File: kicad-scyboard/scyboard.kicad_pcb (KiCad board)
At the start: 2 copper layers, 149 x 95.4 mm, 92 parts

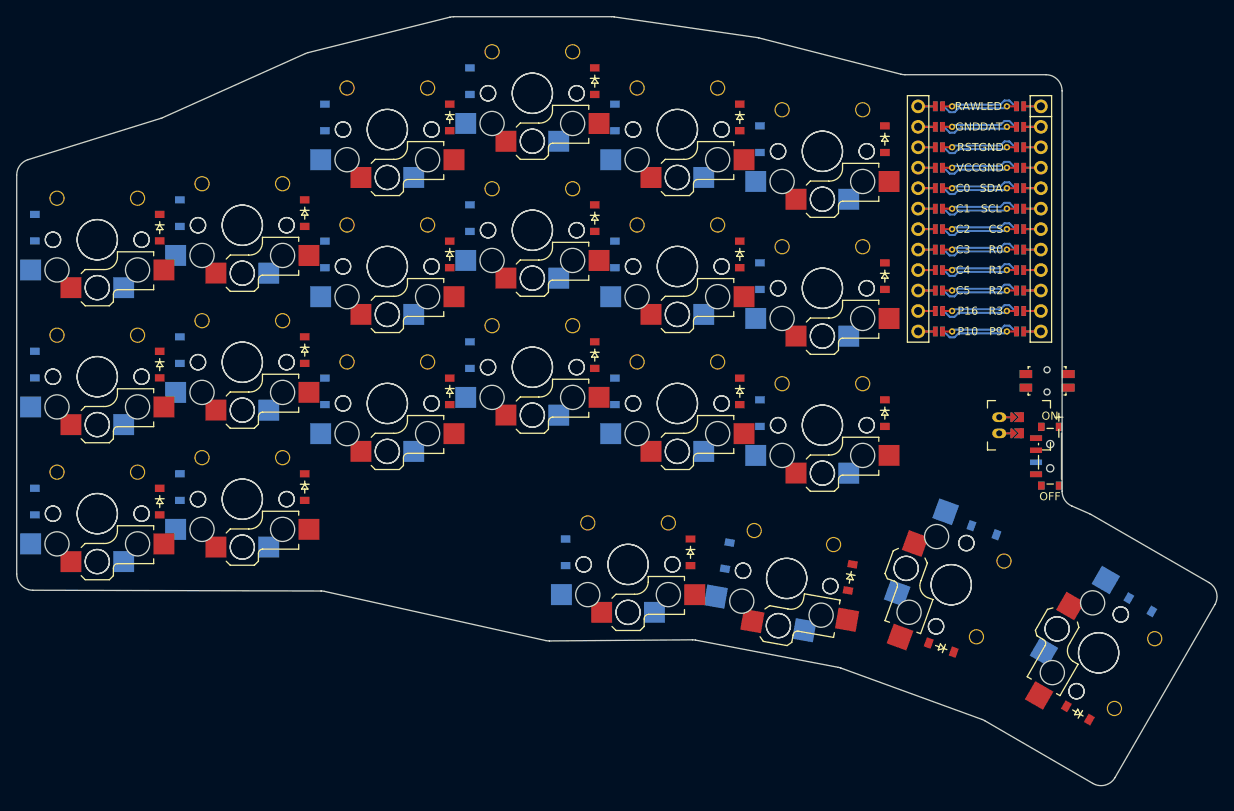
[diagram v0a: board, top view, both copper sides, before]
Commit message: Update KiCad
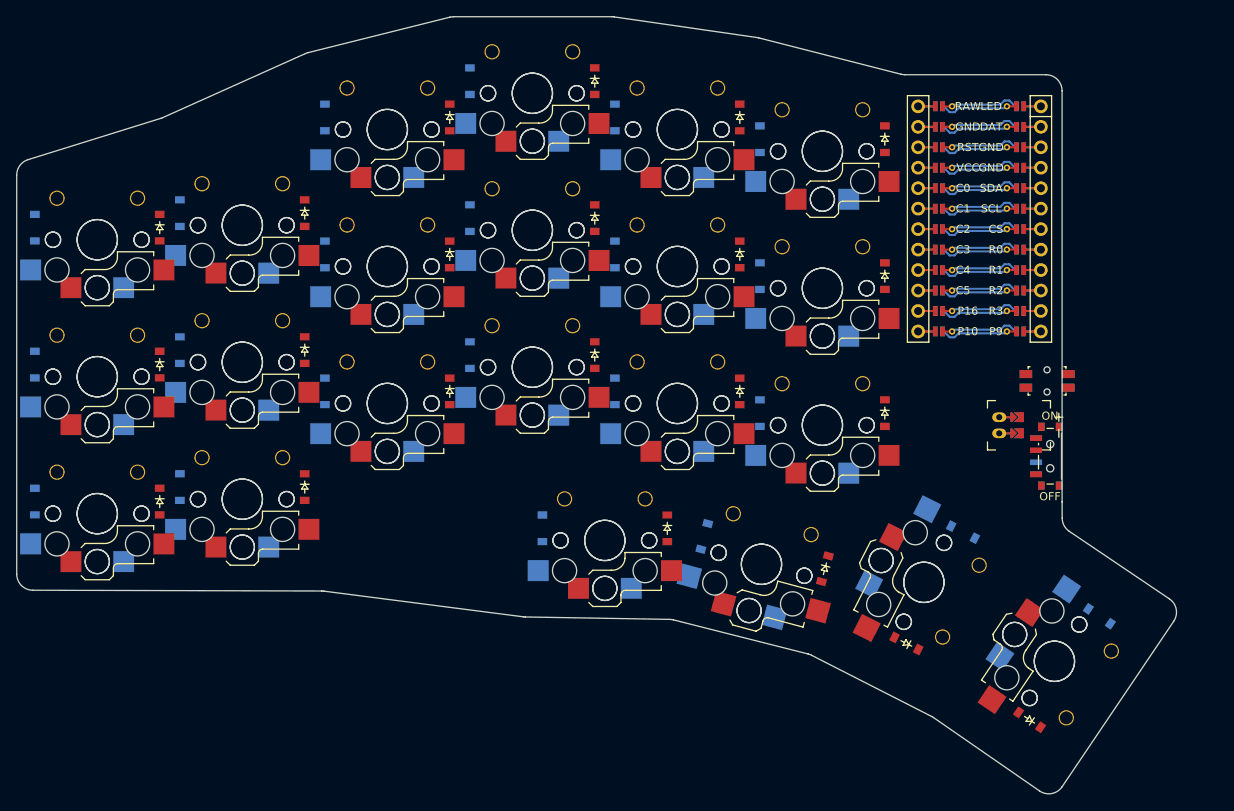
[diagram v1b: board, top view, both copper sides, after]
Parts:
- moved D44 6.06 mm to (165.7, 125.6), turned to -214 degrees
- moved S22 5.59 mm to (168.8, 118.3), turned to 56 degrees
- moved S44 5.59 mm to (168.8, 118.3), turned to 56 degrees
- moved D22 5.28 mm to (174.4, 112.7), turned to -214 degrees
- moved D43 4.36 mm to (150.4, 116.1), turned to -207 degrees
- moved D19 4.14 mm to (105.2, 101.8)
- moved D41 4.14 mm to (120.8, 101.8)
- moved S19 4.14 mm to (113.0, 103.3)
- moved S41 4.14 mm to (113.0, 103.3)
- moved D20 3.72 mm to (125.3, 102.8), turned to -105 degrees
- moved S20 3.59 mm to (132.4, 106.3), turned to 165 degrees
- moved S42 3.59 mm to (132.4, 106.3), turned to 165 degrees
- moved S21 3.40 mm to (152.6, 108.5), turned to 63 degrees
- moved S43 3.40 mm to (152.6, 108.5), turned to 63 degrees
- moved D42 3.32 mm to (140.3, 106.8), turned to -105 degrees
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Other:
- board size 149 x 95.4 mm -> 143.9 x 96.5 mm
